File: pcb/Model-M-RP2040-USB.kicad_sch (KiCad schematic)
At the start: 17 parts, among them J1 Leds, J2 Rows, J3 Columns, J4 USB-C, Q1 2N7002, SW1 SWITCH, U1 74HC589, U2 USBLC6-2SC6, U3 74HC589

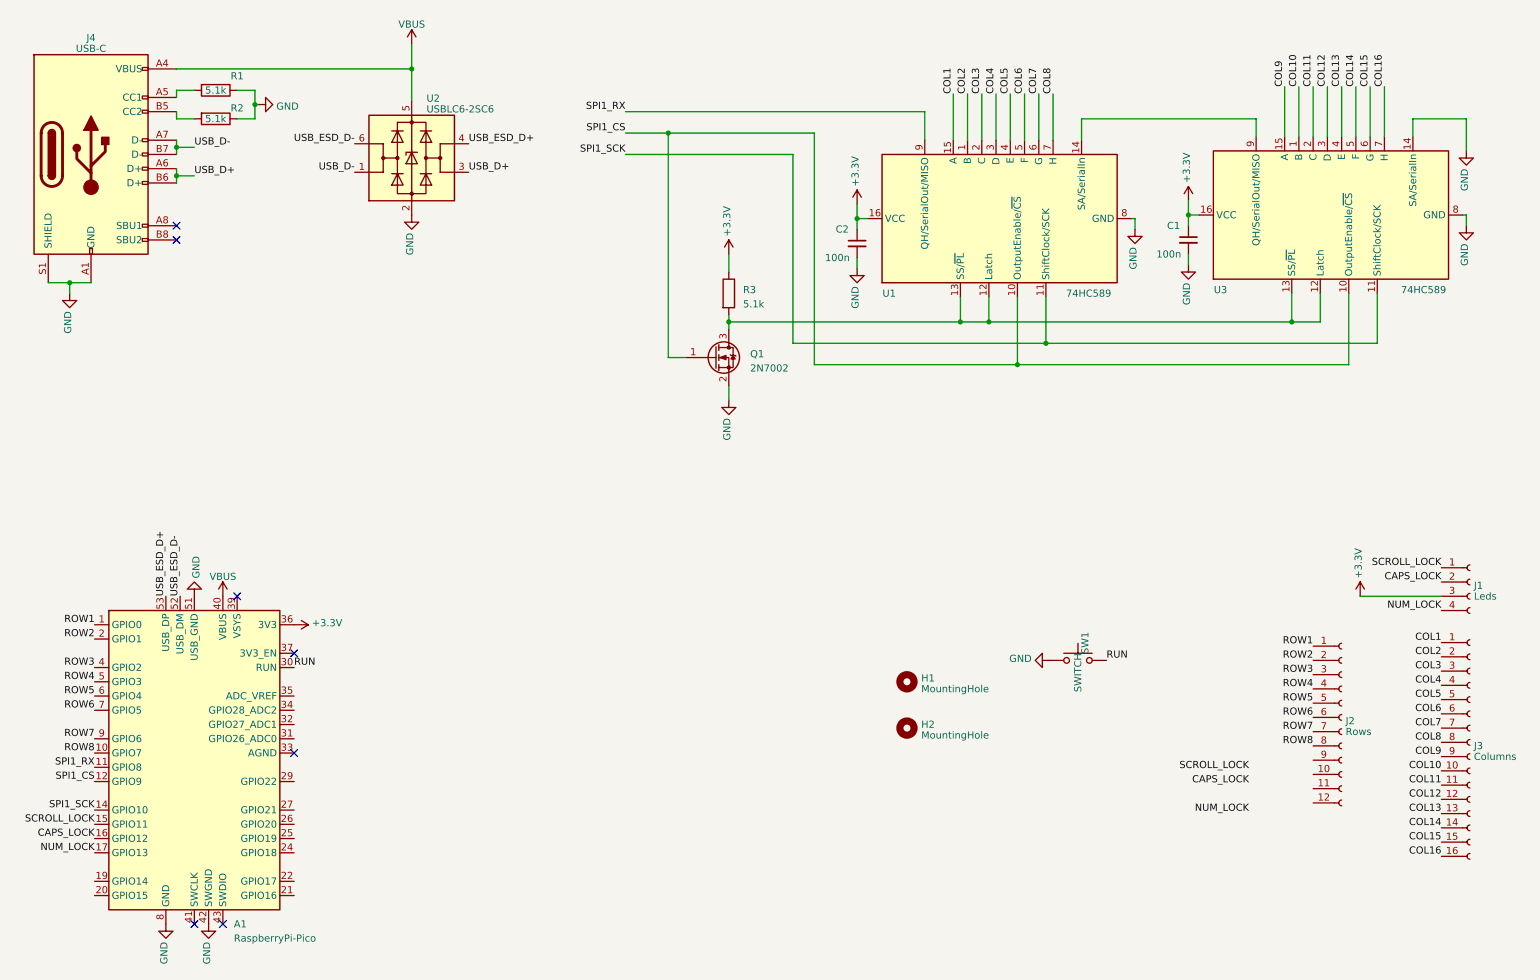
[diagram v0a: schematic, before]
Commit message: Rev 0.2
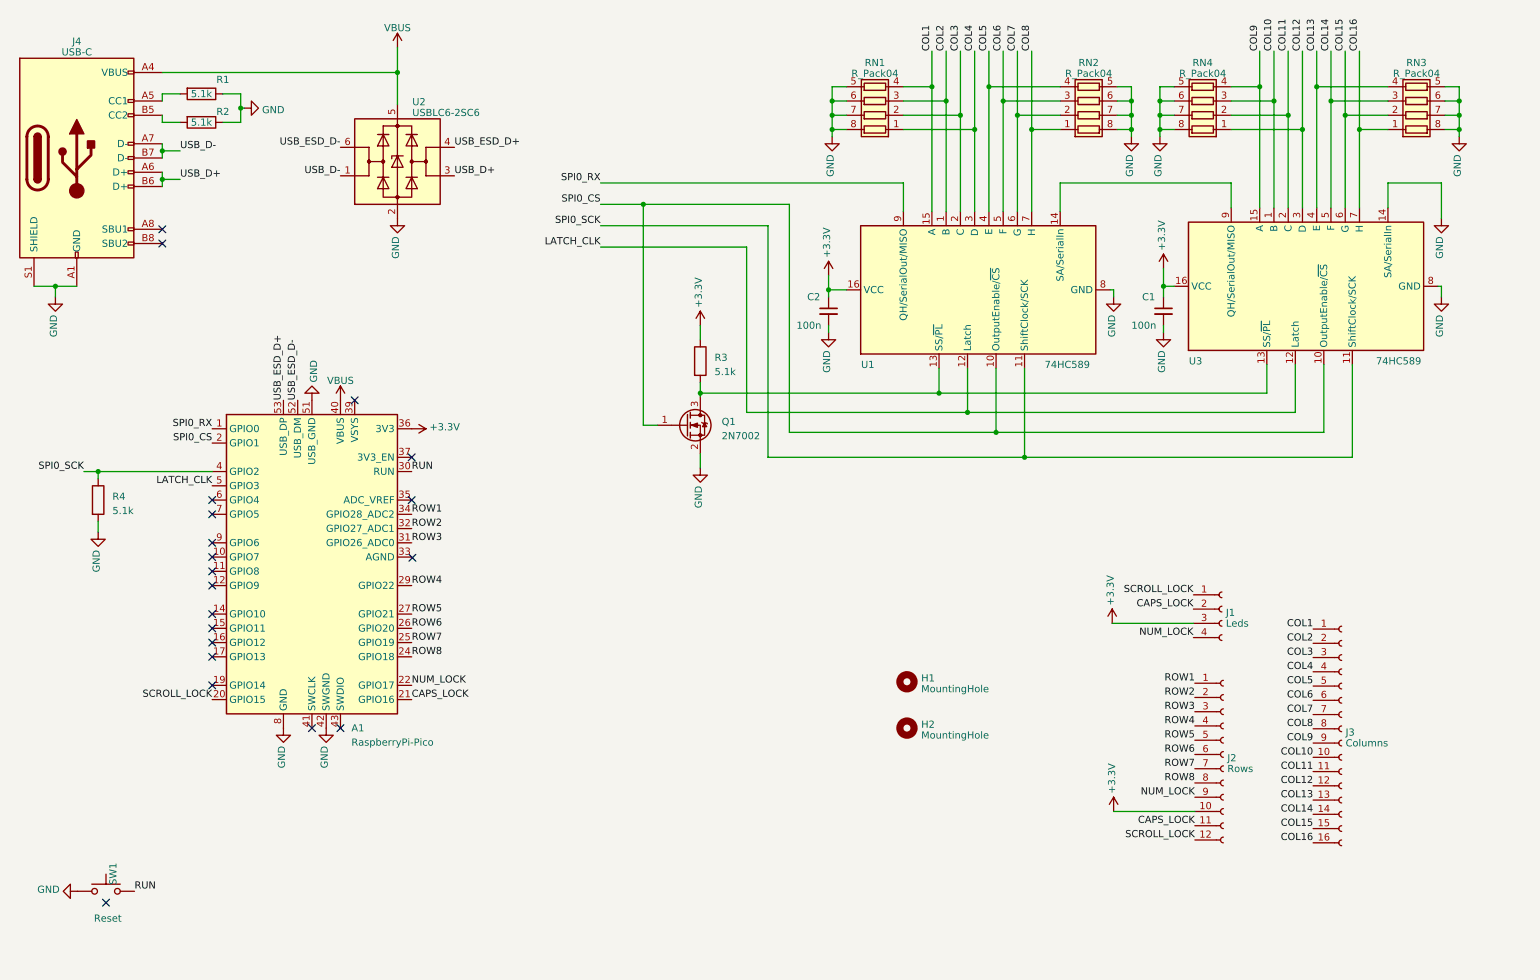
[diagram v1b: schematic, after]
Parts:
- added R4: 5.1k, Resistor_SMD:R_0603_1608Metric, symbol Device:R
- added RN1, RN2, RN3, RN4: R_Pack04, Resistor_SMD:R_Array_Convex_4x0603, symbol Device:R_Pack04
- C1, C2: footprint Capacitor_SMD:C_0603_1608Metric_Pad1.08x0.95mm_HandSolder -> Capacitor_SMD:C_0603_1608Metric
- J2: footprint Connector_PinSocket_2.54mm:PinSocket_1x16_P2.54mm_Vertical -> Connector_PinSocket_2.54mm:PinSocket_1x12_P2.54mm_Vertical
- J3: footprint Connector_PinSocket_2.54mm:PinSocket_1x12_P2.54mm_Vertical -> Connector_PinSocket_2.54mm:PinSocket_1x16_P2.54mm_Vertical
- R3: footprint Resistor_SMD:R_0612_1632Metric_Pad1.18x3.40mm_HandSolder -> Resistor_SMD:R_0603_1608Metric
- SW1: value SWITCH -> Reset; JLC Basic N -> (none); LCSC C589221 -> (none); MPN  ST-1194 -> (none); Manufacturer RI SHENG -> (none); Substitute N -> (none)
- U1, U3: footprint Package_SO:TSSOP-16_4.4x5mm_P0.65mm -> Package_SO:SOIC-16_3.9x9.9mm_P1.27mm
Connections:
- net +3V3: now also J2.10 (Pin_10)
- net CAPS_LOCK: now also A1.21 (GPIO16), J2.11 (Pin_11); no longer A1.16 (GPIO12)
- net COL1: now also RN1.4 (R4.1)
- net COL10: now also RN4.3 (R3.1)
- net COL11: now also RN4.2 (R2.1)
- net COL12: now also RN4.1 (R1.1)
- net COL13: now also RN3.4 (R4.1)
- net COL14: now also RN3.3 (R3.1)
- net COL15: now also RN3.2 (R2.1)
- net COL16: now also RN3.1 (R1.1)
- net COL2: now also RN1.3 (R3.1)
- net COL3: now also RN1.2 (R2.1)
- net COL4: now also RN1.1 (R1.1)
- net COL5: now also RN2.4 (R4.1)
- net COL6: now also RN2.3 (R3.1)
- net COL7: now also RN2.2 (R2.1)
- net COL8: now also RN2.1 (R1.1)
- net COL9: now also RN4.4 (R4.1)
- net GND: now also R4.2, RN1.5 (R4.2), RN1.6 (R3.2), RN1.7 (R2.2), RN1.8 (R1.2), RN2.5 (R4.2), RN2.6 (R3.2), RN2.7 (R2.2), RN2.8 (R1.2), RN3.5 (R4.2), RN3.6 (R3.2), RN3.7 (R2.2), RN3.8 (R1.2), RN4.5 (R4.2), RN4.6 (R3.2), RN4.7 (R2.2), RN4.8 (R1.2)
- net NUM_LOCK: now also A1.22 (GPIO17), J2.9 (Pin_9); no longer A1.17 (GPIO13)
- net ROW1: now also A1.34 (GPIO28_ADC2); no longer A1.1 (GPIO0)
- net ROW2: now also A1.32 (GPIO27_ADC1); no longer A1.2 (GPIO1)
- net ROW3: now also A1.31 (GPIO26_ADC0); no longer A1.4 (GPIO2)
- net ROW4: now also A1.29 (GPIO22); no longer A1.5 (GPIO3)
- net ROW5: now also A1.27 (GPIO21); no longer A1.6 (GPIO4)
- net ROW6: now also A1.26 (GPIO20); no longer A1.7 (GPIO5)
- net ROW7: now also A1.25 (GPIO19); no longer A1.9 (GPIO6)
- net ROW8: now also A1.24 (GPIO18); no longer A1.10 (GPIO7)
- net SCROLL_LOCK: now also A1.20 (GPIO15), J2.12 (Pin_12); no longer A1.15 (GPIO11)
- net at Q1.3 (D), R3.2, U1.13 (SS/~{PL})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: no longer U1.12 (Latch), U3.12 (Latch)
- net SPI1_CS renamed SPI0_CS
- net SPI0_CS: now also A1.2 (GPIO1); no longer A1.12 (GPIO9)
- net SPI1_RX: no longer names the net of A1.11 (GPIO8)
- net SPI1_RX: no longer U1.9 (QH/SerialOut/MISO)
- net SPI1_SCK renamed SPI0_SCK
- net SPI0_SCK: now also A1.4 (GPIO2), R4.1; no longer A1.14 (GPIO10)
- new net LATCH_CLK: A1.5 (GPIO3), U1.12 (Latch), U3.12 (Latch)
- new net SPI0_RX: A1.1 (GPIO0), U1.9 (QH/SerialOut/MISO)
- no-connect marks 7 -> 20
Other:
- moved on the sheet: A1, C1, C2, J1, J2, J3, J4, Q1, R1, R2, R3, SW1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
